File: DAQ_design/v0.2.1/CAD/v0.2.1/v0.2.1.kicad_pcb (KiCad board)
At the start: 2 copper layers, 100 x 80 mm, 37 parts, among them J1 Screw_Terminal_01x04, U1 Teensy4.0, U2 L293D, U3 PC817, U5 PC817, U6 PC817, U7 74HC165

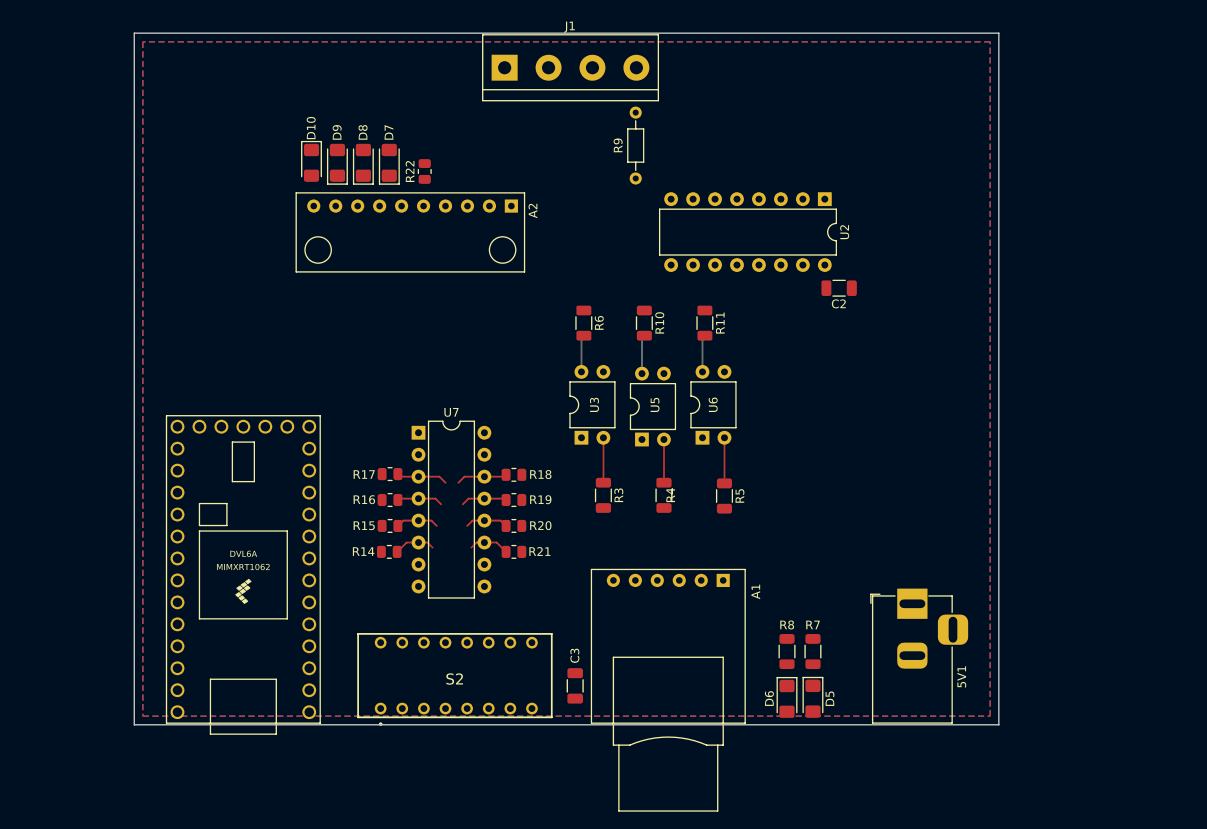
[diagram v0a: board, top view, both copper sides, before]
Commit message: figuring out battery
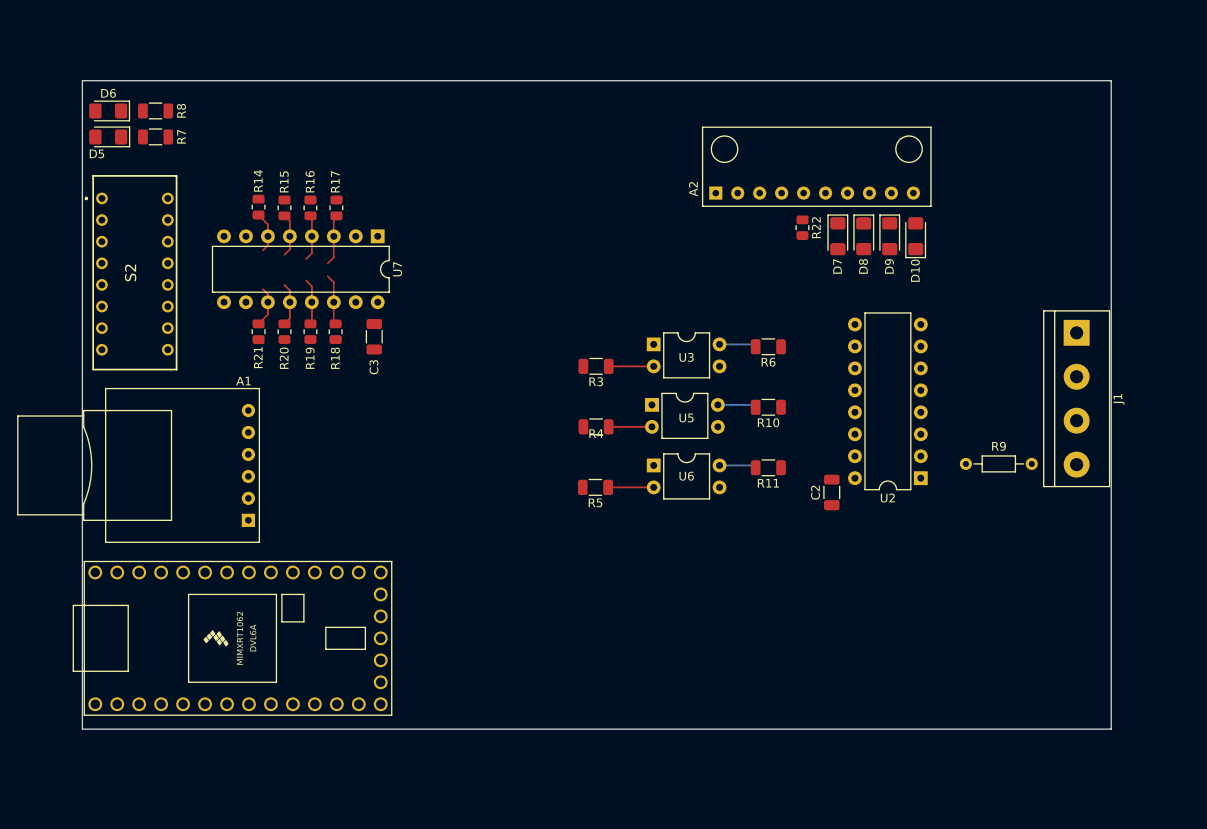
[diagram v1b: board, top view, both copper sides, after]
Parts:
- removed 5V1: Barrel_Jack, Connector_BarrelJack:BarrelJack_Horizontal
- moved D5 104.2 mm to (97.0, 62.0), turned to 180 degrees
- moved D6 103.9 mm to (97.0, 59.0), turned to 180 degrees
- moved R7 96.6 mm to (102.5, 62.0), turned to 180 degrees
- moved R8 96.1 mm to (102.5, 59.0), turned to 180 degrees
- moved J1 72.9 mm to (209.0, 84.7), turned to -90 degrees
- moved D10 70.4 mm to (190.4, 73.5), turned to 90 degrees
- moved S2 67.2 mm to (96.3, 69.1), turned to -90 degrees
- moved D9 64.4 mm to (187.4, 73.5), turned to -90 degrees
- moved R9 61.2 mm to (203.8, 99.8), turned to 180 degrees
- moved D8 58.5 mm to (184.4, 73.5), turned to -90 degrees
- moved A1 55.4 mm to (113.2, 106.3), turned to 180 degrees
- moved D7 52.6 mm to (181.4, 73.5), turned to -90 degrees
- moved C3 46.6 mm to (127.8, 85.1), turned to 90 degrees
- moved R22 44.2 mm to (177.3, 72.5), turned to -90 degrees
- moved R14 42.7 mm to (114.4, 70.1), turned to -90 degrees
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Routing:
- removed copper zone on B.Cu, net GND
- removed copper zone on F.Cu, net GNDD
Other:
- board size 100 x 80 mm -> 119 x 75 mm

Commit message: bad traces
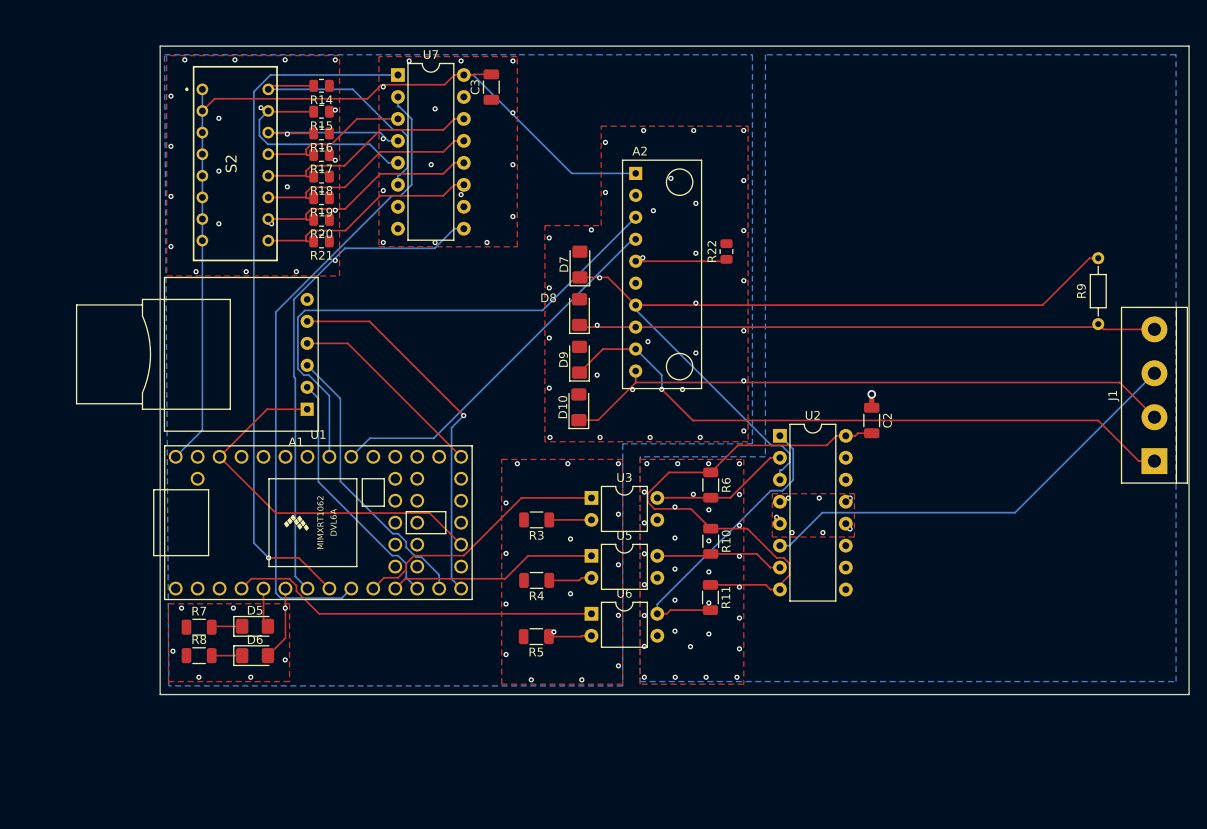
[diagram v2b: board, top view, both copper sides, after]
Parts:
- moved D6 65.3 mm to (114.0, 122.0), turned to 0 degrees
- moved R8 63.2 mm to (107.5, 122.0), turned to 0 degrees
- moved D5 59.1 mm to (114.0, 118.6), turned to 0 degrees
- moved R7 56.9 mm to (107.5, 118.7), turned to 0 degrees
- moved D10 43.7 mm to (151.4, 93.3)
- moved D9 38.6 mm to (151.5, 87.8), turned to 90 degrees
- moved D8 34.0 mm to (151.5, 82.3), turned to 90 degrees
- moved C3 31.9 mm to (141.3, 56.2)
- moved D7 30.0 mm to (151.5, 76.8), turned to 90 degrees
- moved U3 19.2 mm to (152.9, 103.8)
- moved R3 19.0 mm to (146.5, 106.3)
- moved R4 19.0 mm to (146.5, 113.3)
- moved U5 18.8 mm to (152.9, 110.5)
- moved U7 18.8 mm to (130.5, 54.8), turned to 0 degrees
- moved U6 18.6 mm to (152.9, 117.2)
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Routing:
- net VDD: track 0.00 -> 103.5 mm
- net EX+: track 0.00 -> 92.4 mm
- net DIPLAT: track 0.00 -> 80.6 mm, vias 0 -> 1
- net DIPCP: track 0.00 -> 74.7 mm
- net IN2: track 0.00 -> 74.0 mm, vias 0 -> 1
- net IN3: track 0.00 -> 71.4 mm
- net IN1: track 0.00 -> 67.0 mm
- net ADC_SCL: track 0.00 -> 61.8 mm
- net VPP: track 0.00 -> 61.1 mm
- net DIPDAT: track 0.00 -> 57.1 mm
- net EX-: track 0.00 -> 51.6 mm
- net +3.3V: track 0.00 -> 44.6 mm
- net SDMISO: track 0.00 -> 43.7 mm, vias 0 -> 1
- net ADC_SDA: track 0.00 -> 43.3 mm
- net EN: track 0.00 -> 43.0 mm
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- added copper zone on B.Cu, net GND
- added copper zone on F.Cu, net GND
- added copper zone on B.Cu, net GNDD
- added copper zone on F.Cu, net GNDD
